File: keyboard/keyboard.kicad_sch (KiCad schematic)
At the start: 61 parts, among them J1 Conn_02x12_Odd_Even, SW1 true video, SW10 8, SW11 9, SW12 0, SW13 Break, SW14 delete, SW15 q, SW16 w, SW17 e, SW18 r, SW19 t, SW2 inverted video, SW20 y, SW21 u, SW22 i, SW23 o, SW24 p, SW25 graph, SW26 extended mode, SW27 edit, SW28 a, SW29 s, SW3 1, SW30 d, SW31 f, SW32 g, SW33 h, SW34 j, SW35 k, SW36 l, SW37 enter, SW38 caps shift left, SW39 caps lock, SW4 2, SW40 z, SW41 x, SW42 c, SW43 v, SW44 b, SW45 n, SW46 m, SW47 dot, SW48 caps shift right, SW49 symbol shift left, SW5 3, SW50 semicolon, SW51 quotes, SW52 left, SW53 right, SW54 left space, SW55 right space, SW56 up, SW57 down, SW58 comma, SW59 symbol shift right, SW6 4, SW60 rus-lat, SW7 5, SW8 6, SW9 7

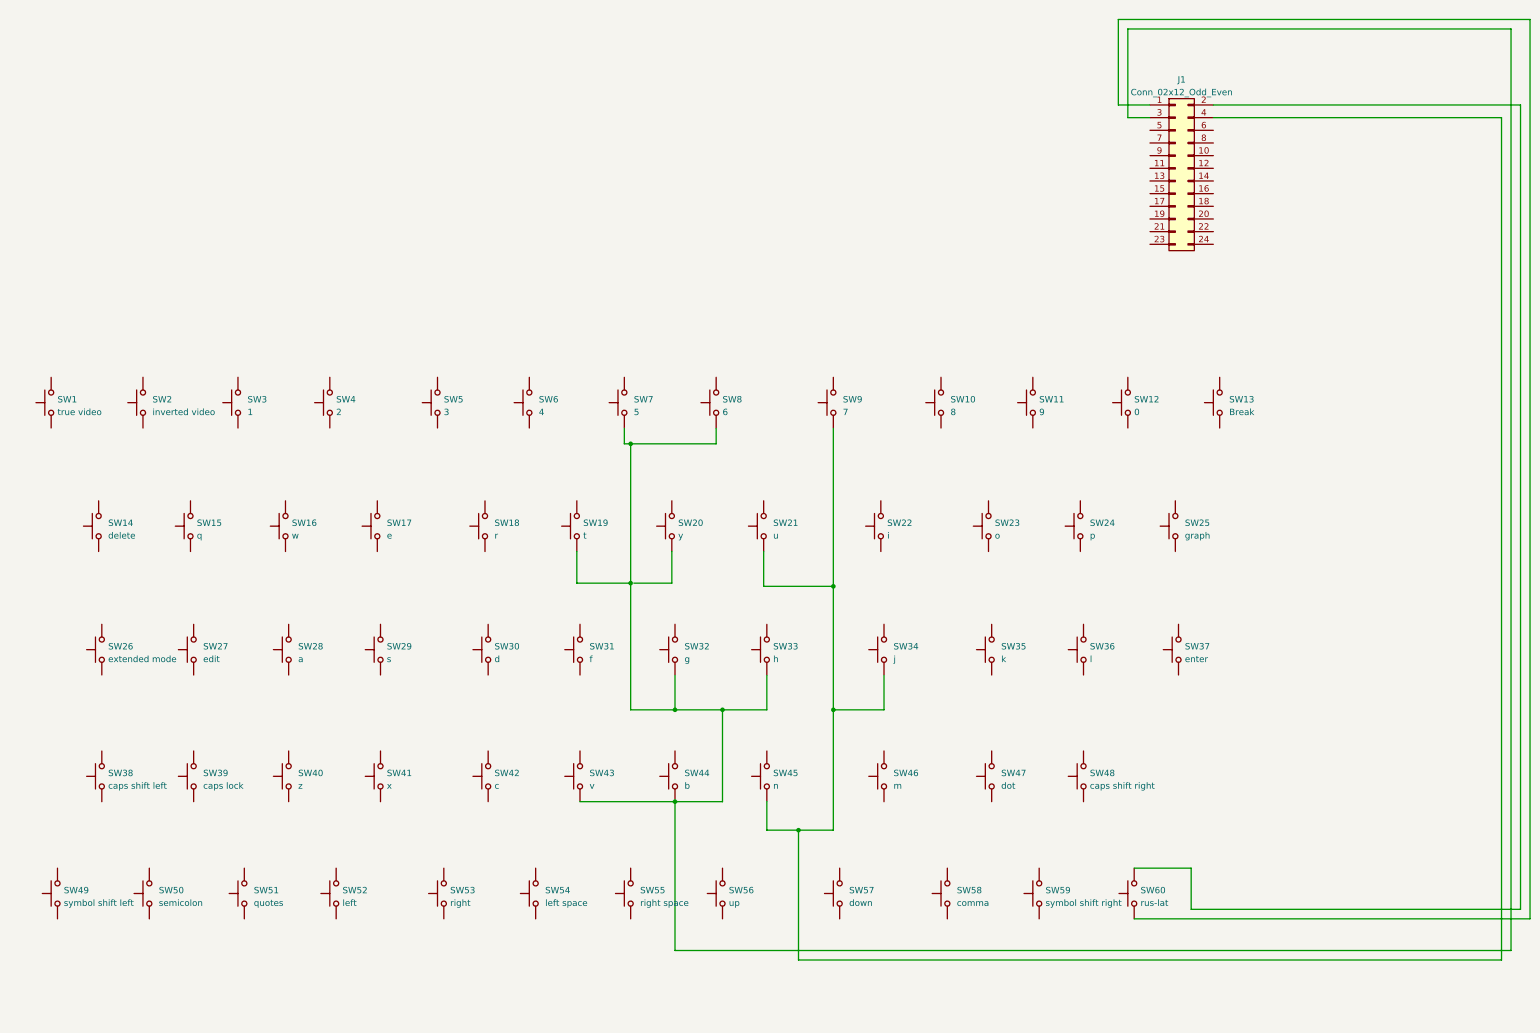
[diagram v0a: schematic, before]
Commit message: Updade
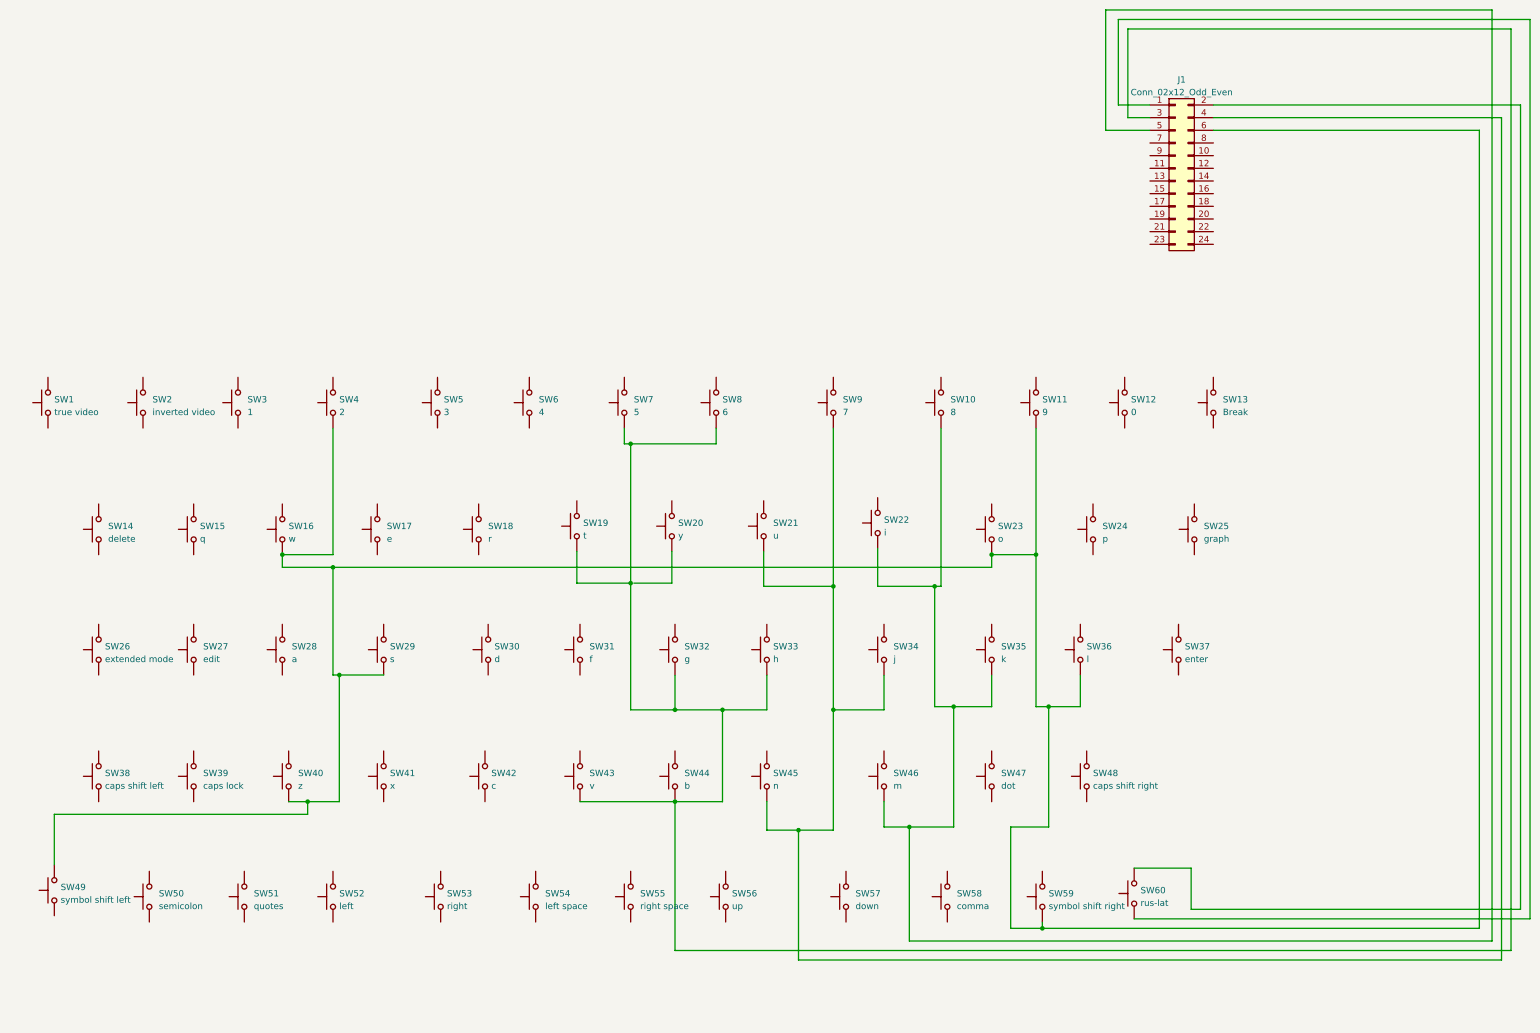
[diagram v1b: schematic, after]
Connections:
- net at SW35.1: now also J1.5 (Pin_5), SW10.1, SW22.1, SW46.1
- net at SW40.1: now also J1.6 (Pin_6), SW11.1, SW16.1, SW23.1, SW29.1, SW36.1, SW4.1, SW49.2, SW59.1
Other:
- moved on the sheet: SW1, SW11, SW12, SW13, SW14, SW15, SW16, SW17, SW18, SW22, SW23, SW24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

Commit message: Update 20092023
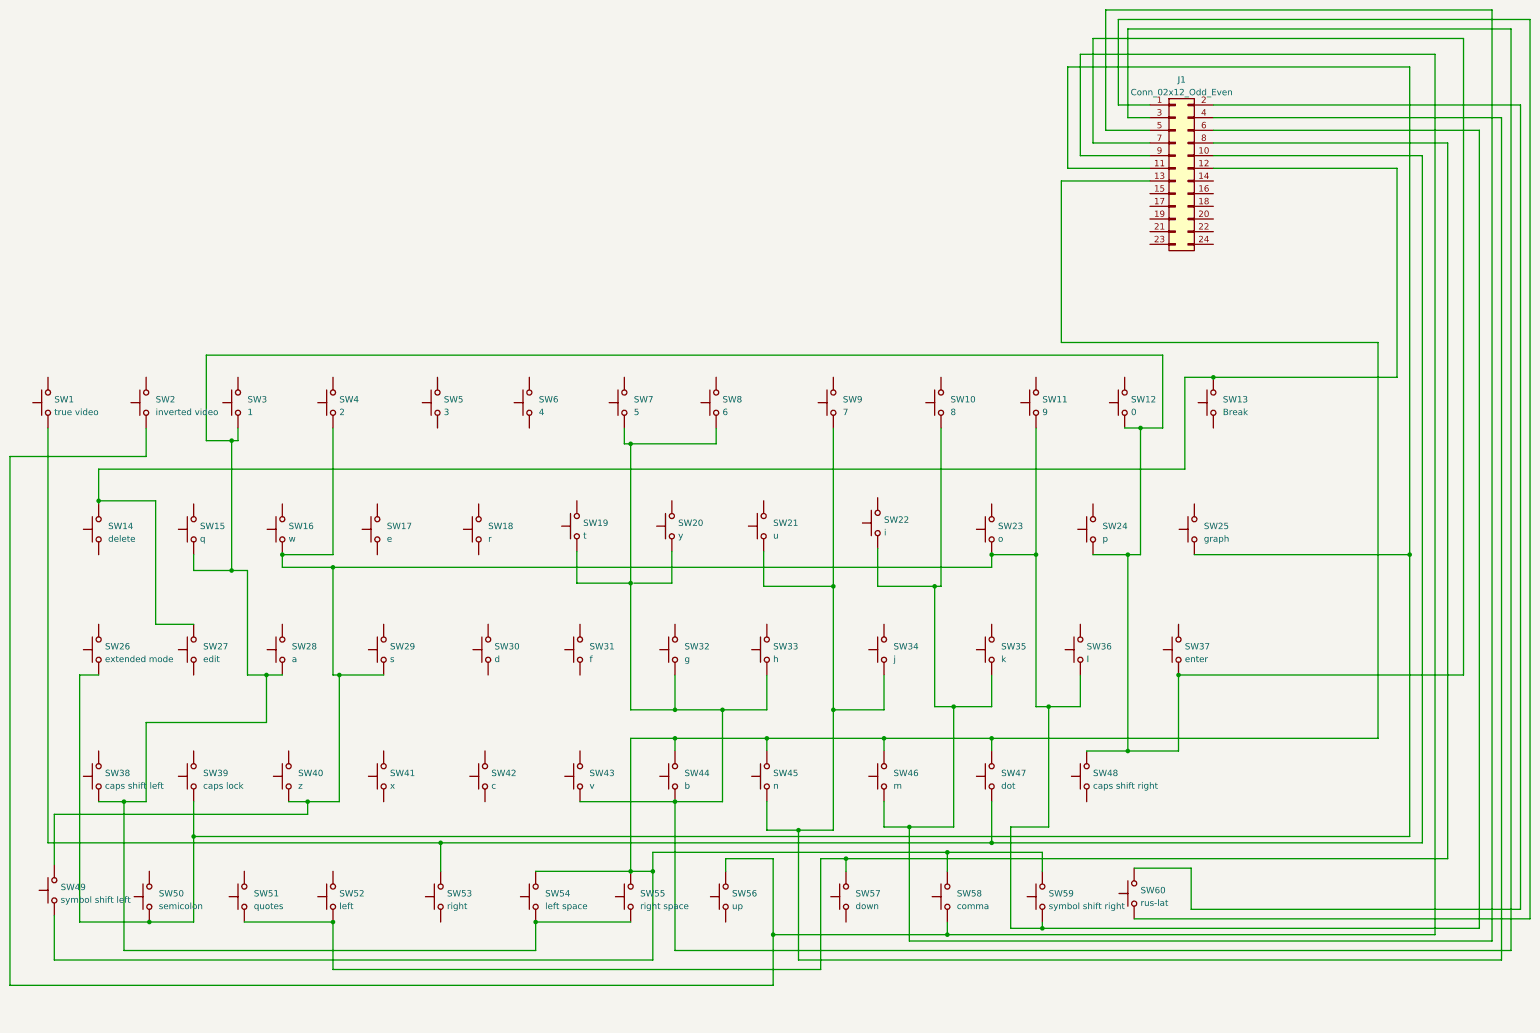
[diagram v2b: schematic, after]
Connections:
- net at SW28.1: now also J1.7 (Pin_7), SW12.1, SW15.1, SW24.1, SW3.1, SW37.1, SW38.1, SW48.2, SW54.1, SW55.1
- net at SW57.2: now also J1.8 (Pin_8), SW51.1, SW52.1
- net at SW47.1: now also J1.10 (Pin_10), SW1.1, SW53.2
- net at SW47.2: now also J1.13 (Pin_13), SW44.2, SW45.2, SW46.2, SW49.1, SW54.2, SW55.2, SW58.2, SW59.2
- net at SW58.1: now also J1.9 (Pin_9), SW2.1, SW56.2
- net at SW14.2: now also J1.12 (Pin_12), SW13.2, SW27.2
- net at SW25.1: now also J1.11 (Pin_11), SW26.1, SW39.1, SW50.1
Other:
- moved on the sheet: SW2
